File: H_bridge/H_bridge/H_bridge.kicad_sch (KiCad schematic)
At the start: 17 parts, among them J1 Screw_Terminal_01x02, J2 Screw_Terminal_01x06, J3 Pins_02x10_P1.27mm_TH, U1 VNH7040AYTR

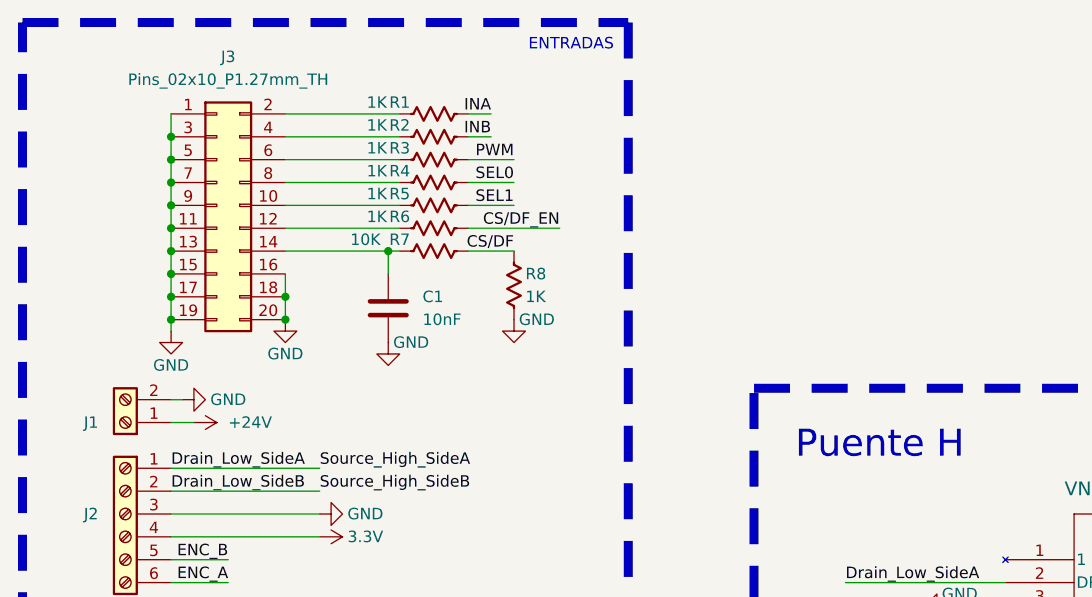
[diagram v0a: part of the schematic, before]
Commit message: puente H, Done
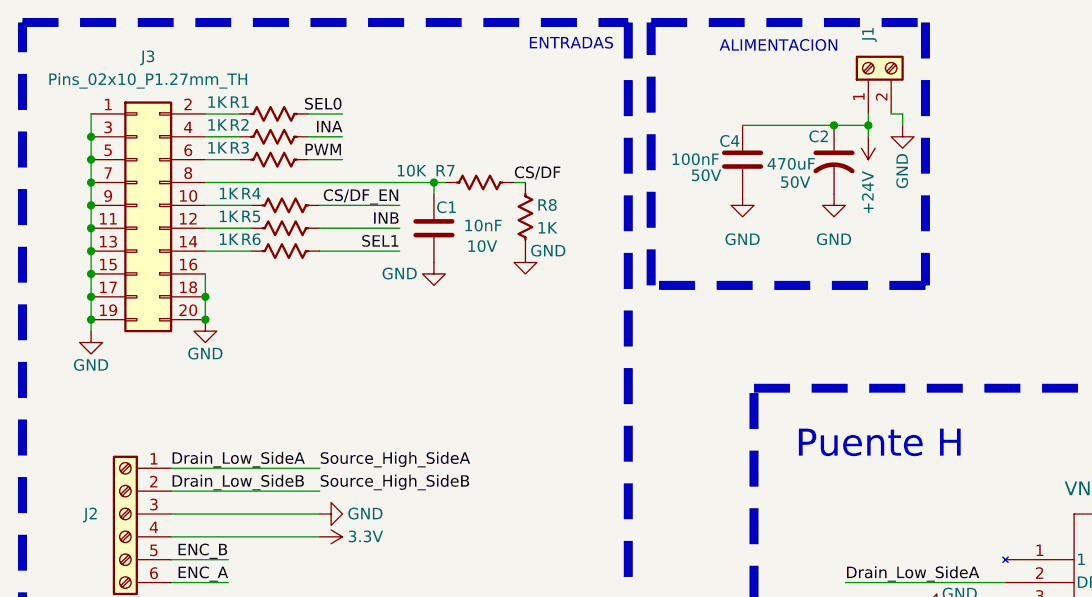
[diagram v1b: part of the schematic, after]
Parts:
- added C2: 470uF, Capacitor_SMD:CP_Elec_10x14.3, symbol Device:C_US
- added C4: 100nF, PCM_Capacitor_SMD_AKL:C_0805_2012Metric, symbol PCM_Capacitor_AKL:C_0805
- C1: V (none) -> 10V
- U1: footprint UL_Hbridge:POWERSSO-36TP_STM-M -> UL_Full_H_Bridge_SMD:POWERSSO-36TP_STM-M
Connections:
- net +24V: now also C2.1, C4.1
- net CS/DF_EN: now also R4.2; no longer R6.2
- net GND: now also C2.2, C4.2
- net INA: now also R2.2; no longer R1.2
- net INB: now also R5.2; no longer R2.2
- net SEL0: now also R1.2; no longer R4.2
- net SEL1: now also R6.2; no longer R5.2
- net at R5.1: now also J3.12; no longer J3.10
- net at C1.1, R7.1: now also J3.8; no longer J3.14
- net at R4.1: now also J3.10; no longer J3.8
- net at R6.1: now also J3.14; no longer J3.12
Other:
- note added: "ALIMENTACION"
- moved on the sheet: C1, J1, J3, R1, R2, R3, R4, R5, R6, R7, R8
